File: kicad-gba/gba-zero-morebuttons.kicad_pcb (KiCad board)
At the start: 2 copper layers, 130.7 x 72.9 mm, 71 parts, among them J1 SWTCHCRFT_3.5JACK5-JACK-SMD, P1 50_PIN_CON, P3 LINK_CONNECTOR, Q1 BSS138, U1 APX803, U2 NC7WZ16, U3 74LVC2G02, U4 74LVC3G04, U5 LM4875, U6 RPI-ZEROSMD, U7 POWERBOOST-1000C

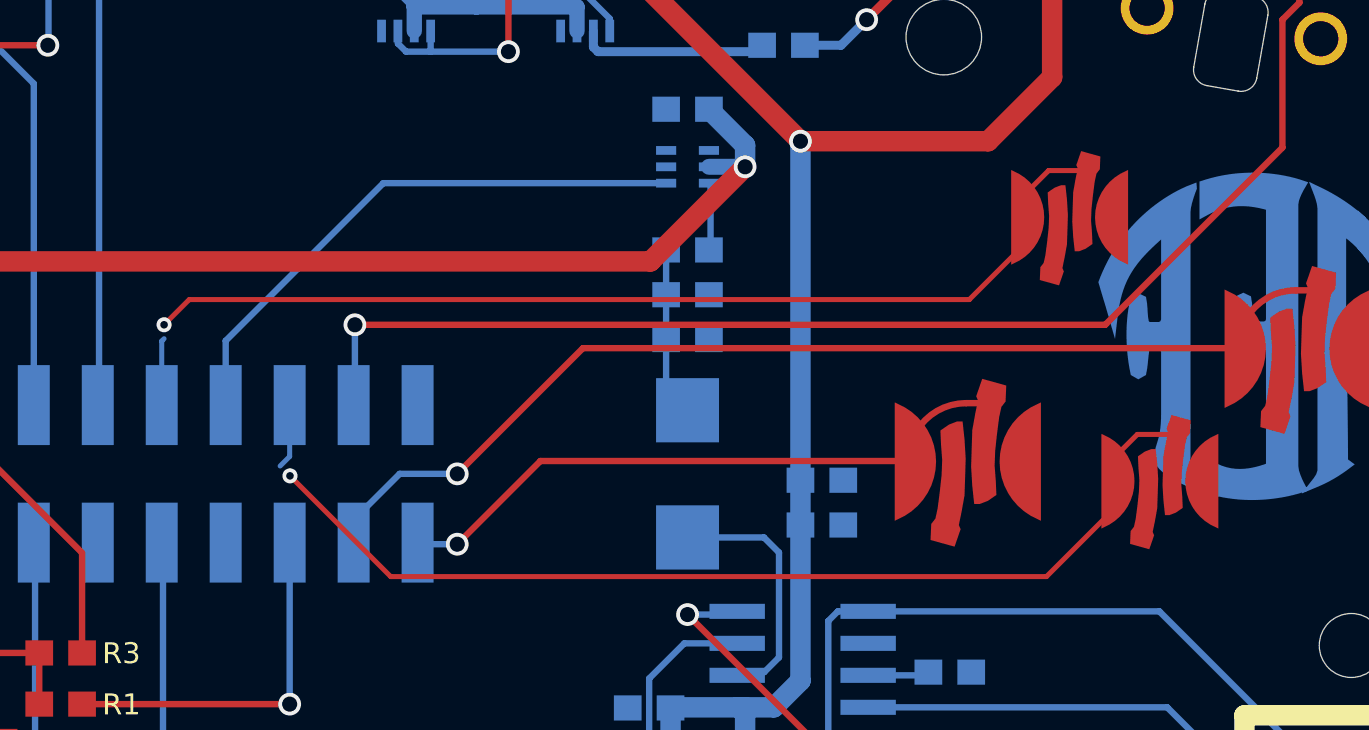
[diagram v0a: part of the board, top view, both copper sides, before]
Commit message: fixed major issue
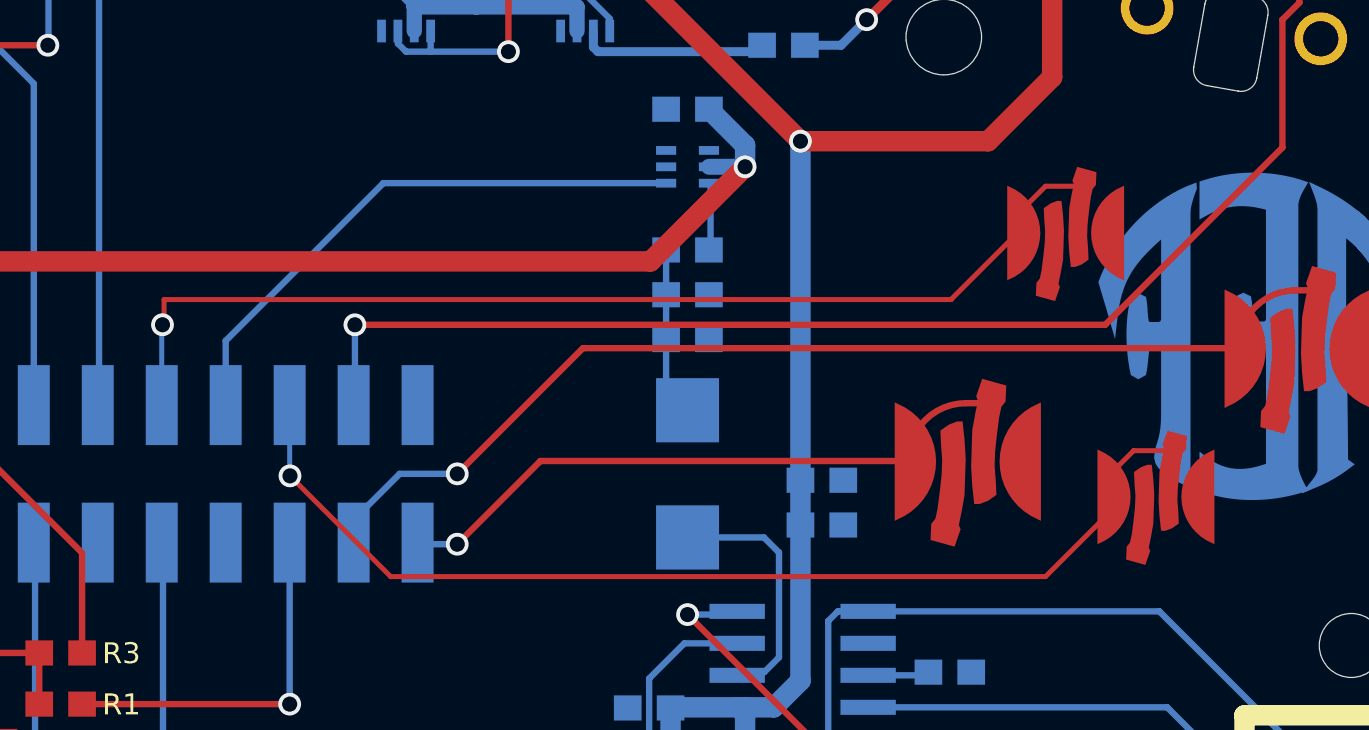
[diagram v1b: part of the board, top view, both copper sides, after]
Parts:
- removed REF**: Val**, gba-zero-morebuttons:XY_BUTTON
- added S7: XY_BUTTON, gba-zero-morebuttons:XY_BUTTON, F.Cu at (200.1, 97.6)
- P2: value (none) -> JST_2PIN
- S5: value Val** -> AB_BUTTON
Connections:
- net AUD_PWM renamed /AUD_PWM
- net BAT renamed Net-(P2-2)
- net BKLT renamed /BKLT
- net BKLT_PWM renamed /BKLT_PWM
- net BTN_A renamed /BTN_A
- net BTN_B renamed /BTN_B
- net BTN_D renamed /BTN_D
- net BTN_L renamed /BTN_L
- net BTN_LS renamed /BTN_LS
- net BTN_R renamed /BTN_R
- net BTN_RS renamed /BTN_RS
- net BTN_SEL renamed /BTN_SEL
- net BTN_STR renamed /BTN_STR
- net BTN_U renamed /BTN_U
- net BYPASS renamed Net-(C10-P$1)
- net LBO renamed /LBO
- net MISO renamed /MISO
- net MOSI renamed /MOSI
- net MOSI_3V renamed /MOSI_3V
- net PWR_EN_RPI renamed /PWR_EN_RPI
- net PWR_SW_SEN renamed /PWR_SW_SEN
- net RING renamed Net-(C13-P$2)
- net RT_INT renamed /RT_INT
- net RXD renamed /RXD
- net SCL renamed /SCL
- net SCLK renamed /SCLK
- net SCLK_3V renamed /SCLK_3V
- net SDA renamed /SDA
- net SENSE renamed Net-(U5-SENSE)
- net TFT_CS_3V renamed /TFT_CS_3V
- net TFT_DC_3V renamed /TFT_DC_3V
- net TFT_RST renamed /TFT_RST
- net TXD renamed /TXD
- net USB renamed /USB
- net VO1 renamed Net-(C13-P$1)
- net VO2 renamed Net-(SP1--)
- net VOL/SD renamed Net-(U5-VOL/~{SD})
- J1 pad 4: (no net) -> unconnected-(J1-Pad4)
- P1 pad 11: (no net) -> unconnected-(P1-VSYNC-Pad11)
- P1 pad 12: (no net) -> unconnected-(P1-HSYNC-Pad12)
- P1 pad 13: (no net) -> unconnected-(P1-DOTCLK-Pad13)
- P1 pad 14: (no net) -> unconnected-(P1-DE-Pad14)
- P1 pad 35: (no net) -> unconnected-(P1-/RD-Pad35)
- P1 pad 39: (no net) -> unconnected-(P1-TE-Pad39)
- R17 pad 2O: (no net) -> unconnected-(R17-Pad2O)
- U2 pad 3: (no net) -> unconnected-(U2-A2-Pad3)
- U2 pad 4: (no net) -> unconnected-(U2-Y2-Pad4)
- U6 pad 31: (no net) -> /BTN_X
- U6 pad 35: (no net) -> /BTN_Y
- U7 pad VS: (no net) -> unconnected-(U7-PadVS)
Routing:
- net (no net): track 78.7 -> 0.00 mm, vias 2 -> 0
- net /BTN_X: track 0.00 -> 43.5 mm, vias 0 -> 1
- net /BTN_Y: track 0.00 -> 42.4 mm, vias 0 -> 1
- net BTN_Y: track 3.77 -> 0.00 mm
- net BTN_X: track 3.73 -> 0.00 mm
